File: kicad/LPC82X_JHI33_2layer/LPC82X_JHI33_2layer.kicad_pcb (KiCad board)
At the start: 2 copper layers, 23.6 x 23.5 mm, 24 parts, among them J1 Conn_02x09_Odd_Even, J2 Conn_02x09_Odd_Even, J3 JTAG_2X05, U1 LPC824M201JHI33, Y1 12MHz

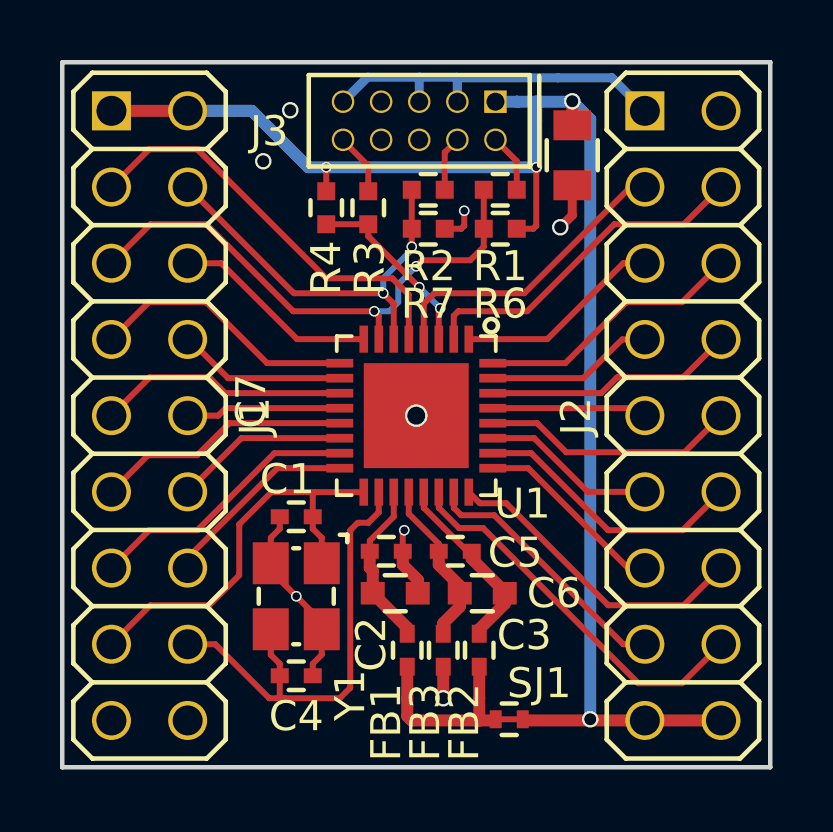
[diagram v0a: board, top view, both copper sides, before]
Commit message: updated pcb and fixed some inconsistencies
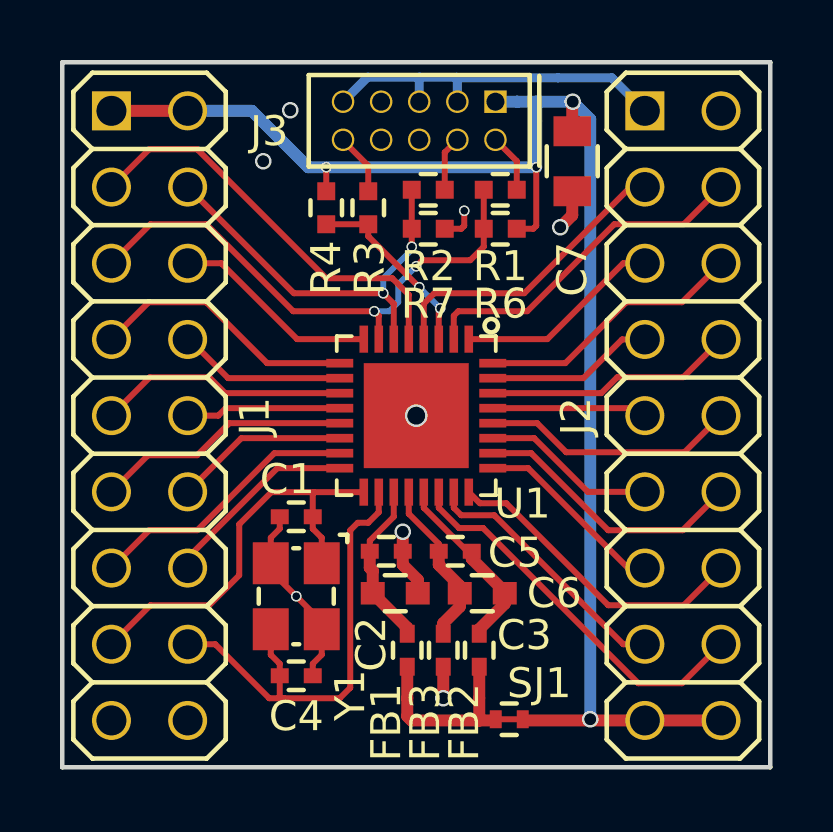
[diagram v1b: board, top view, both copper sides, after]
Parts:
- moved C7 0.20 mm to (94.1, 98.2)
